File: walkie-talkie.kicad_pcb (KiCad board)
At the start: 2 copper layers, 39 x 96 mm, 22 parts, among them U1 ESP32-S3(R8), U10 FS-1540, U11 PJ-327A_5JJ, U12 LIS2DH12TR, U13 MCP73831T-2ACI_OT, U14 ON, U15 AP2112K-3_3TRG1, U16 +, U2 BH-18650-B1BA002, U3 mems-mic, U4 TF-115, U5 SK6812MINI-HS, U6 SK6812MINI-HS, U7 SK6812MINI-HS, U8 SK6812MINI-HS, U9 MAX98357AETE+T

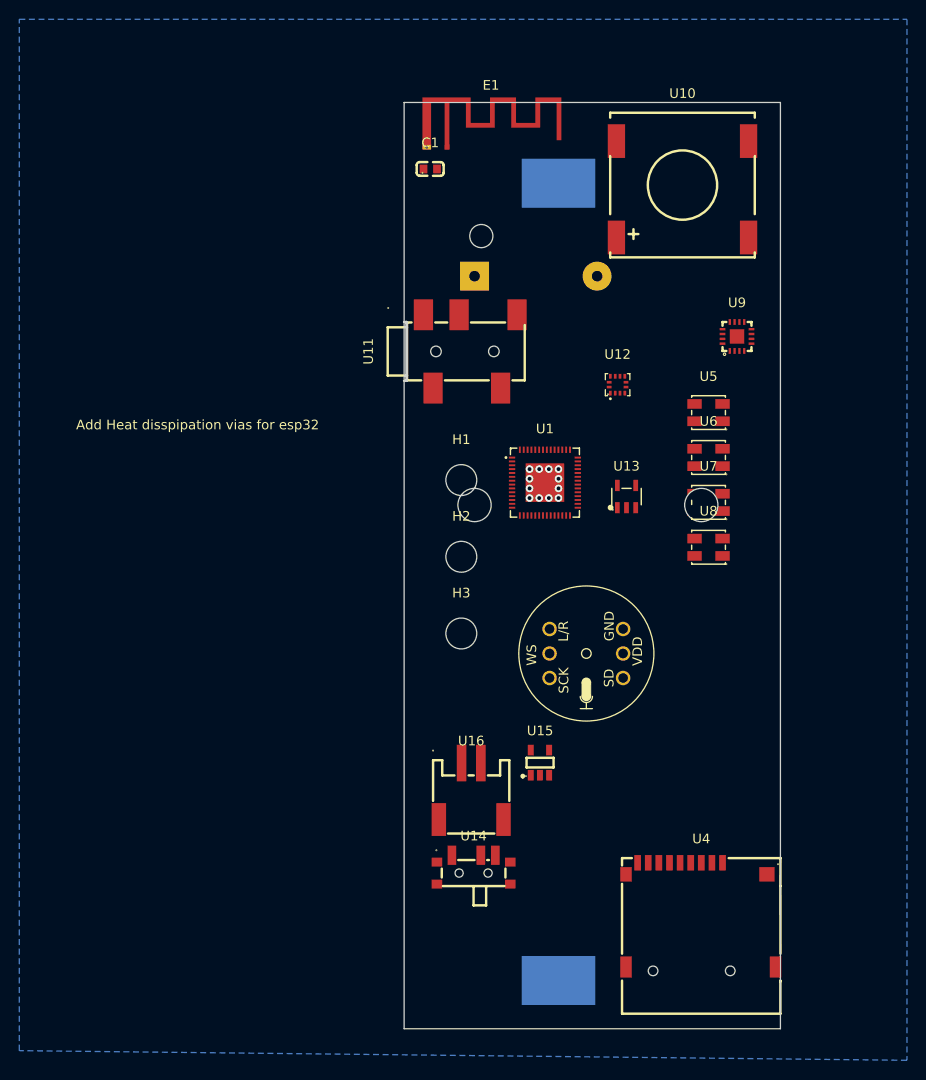
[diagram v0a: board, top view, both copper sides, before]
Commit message: WIP
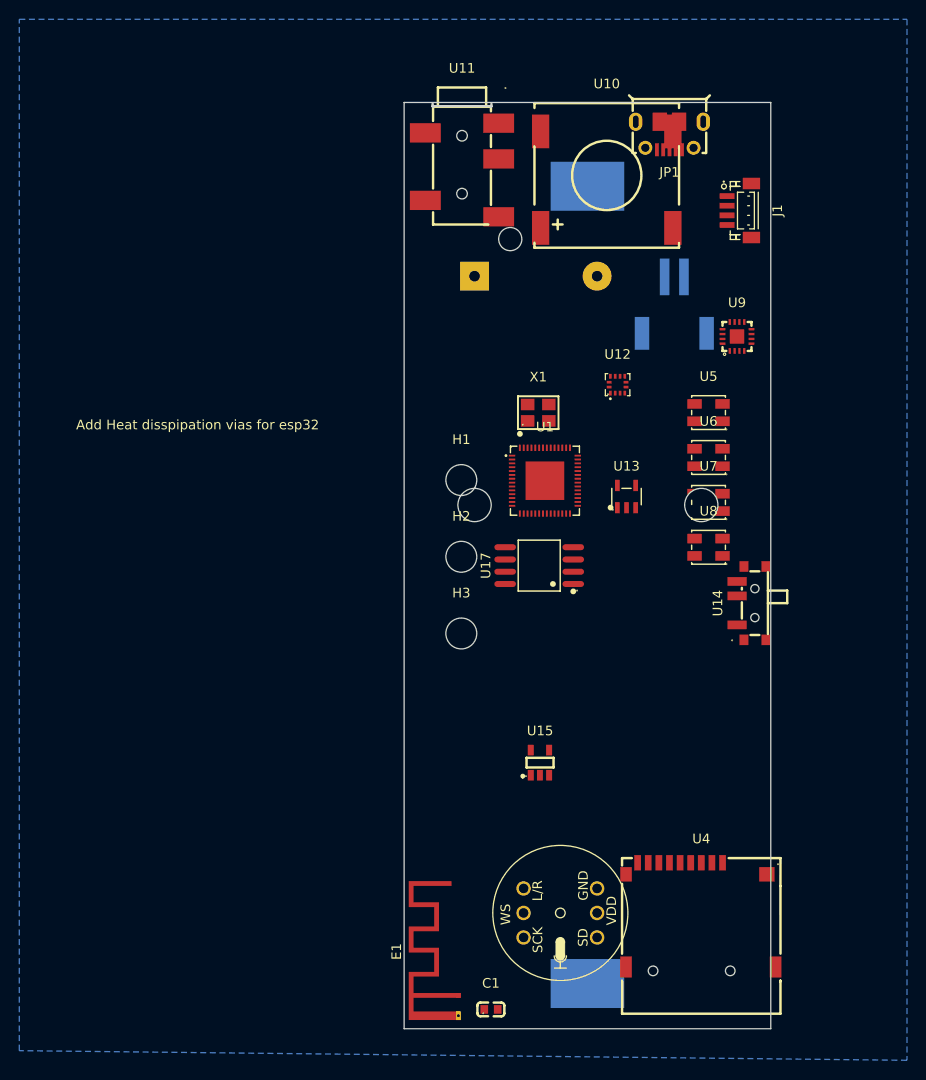
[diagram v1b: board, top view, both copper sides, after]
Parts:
- added J1: I2C, jlc_footprints:CONN-SMD_BM04B-SRSS-TB, F.Cu at (153.7, 45.2)
- added JP1: USB_B_Micro, jlc_footprints:MICRO-USB-SMD_1050171001, F.Cu at (146.5, 37.4)
- added U17: W25Q128JVSIQTR, jlc_footprints:SOIC-8_L5.3-W5.3-P1.27-LS8.0-BL, F.Cu at (133.0, 82.0)
- added X1: X322540MPB4SI, jlc_footprints:OSC-SMD_4P-L3.2-W2.5-BL_SIT8008BI, F.Cu at (132.9, 66.1)
- U16: moved to B.Cu
- moved E1 87.9 mm to (124.6, 126.5), turned to 90 degrees
- moved C1 87.3 mm to (128.0, 128.0)
- moved U16 54.6 mm to (147.0, 55.0), turned to 180 degrees
- moved U14 39.9 mm to (155.0, 85.9), turned to 90 degrees
- moved U3 27.0 mm to (135.2, 118.0)
- moved U11 18.8 mm to (125.0, 41.0), turned to 0 degrees
- moved U10 7.91 mm to (140.0, 42.0)
- moved U2 3.02 mm to (138.0, 84.0)
- moved U1 0.20 mm to (133.6, 73.2)
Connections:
- U1 pad 25: unconnected-(U1-GPIO19-Pad25) -> USB_N
- U1 pad 26: unconnected-(U1-GPIO20-Pad26) -> USB_P
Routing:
- net unconnected-(U1-GND-Pad57): vias 12 -> 0
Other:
- board size 39 x 96 mm -> 38 x 96 mm
